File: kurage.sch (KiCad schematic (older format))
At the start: 106 parts, among them SW1 ESC, SW10 R, SW11 Y, SW12 I, SW13 P, SW14 ], SW15 UNDEFINED2, SW16 CTRL, SW17 A, SW18 D, SW19 G, SW2 Q, SW20 J, SW21 L, SW22 ', SW23 S, SW24 F, SW25 H, SW26 K, SW27 ;, SW28 ENTER, SW29 UNDEFINED3, SW3 E, SW30 LSHIFT, SW31 Z, SW32 C, SW33 B, SW34 M, SW35 ., SW36 RSHIFT, SW37 X, SW38 V, SW39 N, SW4 T, SW40 ,, SW41 /, SW42 UP, SW43 LOWER, SW44 UNDEFINED1, SW45 WIN, SW46 RAISE, SW47 LEFT, SW48 RIGHT, SW49 LSPACE, SW5 U, SW50 RSPACE, SW51 ALT, SW52 DOWN, SW6 O, SW7 [, SW8 BACKSPACE, SW9 W, U1 Elite-C

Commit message: progress
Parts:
- SW1, SW44, SW46: footprint MX_Only:MXOnly-1U-Hotswap -> MX_Only:MXOnly-1.5U-Hotswap
- SW16, SW8: footprint MX_Only:MXOnly-1U-Hotswap -> MX_Only:MXOnly-1.75U-Hotswap
- SW28, SW30: footprint MX_Only:MXOnly-1U-Hotswap -> MX_Only:MXOnly-2.25U-Hotswap
- SW36, SW49: footprint MX_Only:MXOnly-1U-Hotswap -> MX_Only:MXOnly-2U-Hotswap
- SW43: footprint MX_Only:MXOnly-1U-Hotswap -> MX_Only:MXOnly-1.25U-Hotswap
- SW50: footprint MX_Only:MXOnly-1U-Hotswap -> MX_Only:MXOnly-2.75U-Hotswap
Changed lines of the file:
@@
 F 0 "SW44" H 4600 4055 50  0000 C CNN
 F 1 "UNDEFINED1" H 4600 3964 50  0000 C CNN
-F 2 "MX_Only:MXOnly-1U-Hotswap" H 4600 3800 50  0001 C CNN
+F 2 "MX_Only:MXOnly-1.5U-Hotswap" H 4600 3800 50  0001 C CNN
 F 3 "" H 4600 3800 50  0000 C CNN
 	1    4600 3800
@@
 F 0 "SW49" H 4600 4455 50  0000 C CNN
 F 1 "LSPACE" H 4600 4364 50  0000 C CNN
-F 2 "MX_Only:MXOnly-1U-Hotswap" H 4600 4200 50  0001 C CNN
+F 2 "MX_Only:MXOnly-2U-Hotswap" H 4600 4200 50  0001 C CNN
 F 3 "" H 4600 4200 50  0000 C CNN
 	1    4600 4200
@@
 F 0 "SW46" H 6600 4055 50  0000 C CNN
 F 1 "RAISE" H 6600 3964 50  0000 C CNN
-F 2 "MX_Only:MXOnly-1U-Hotswap" H 6600 3800 50  0001 C CNN
+F 2 "MX_Only:MXOnly-1.5U-Hotswap" H 6600 3800 50  0001 C CNN
 F 3 "" H 6600 3800 50  0000 C CNN
 	1    6600 3800
@@
 F 0 "SW28" H 8600 2855 50  0000 C CNN
 F 1 "ENTER" H 8600 2764 50  0000 C CNN
-F 2 "MX_Only:MXOnly-1U-Hotswap" H 8600 2600 50  0001 C CNN
+F 2 "MX_Only:MXOnly-2.25U-Hotswap" H 8600 2600 50  0001 C CNN
 F 3 "" H 8600 2600 50  0000 C CNN
 	1    8600 2600
@@
 F 0 "SW36" H 8600 3255 50  0000 C CNN
 F 1 "RSHIFT" H 8600 3164 50  0000 C CNN
-F 2 "MX_Only:MXOnly-1U-Hotswap" H 8600 3000 50  0001 C CNN
+F 2 "MX_Only:MXOnly-2U-Hotswap" H 8600 3000 50  0001 C CNN
 F 3 "" H 8600 3000 50  0000 C CNN
 	1    8600 3000
@@
 F 0 "SW8" H 9600 1655 50  0000 C CNN
 F 1 "BACKSPACE" H 9600 1564 50  0000 C CNN
-F 2 "MX_Only:MXOnly-1U-Hotswap" H 9600 1400 50  0001 C CNN
+F 2 "MX_Only:MXOnly-1.75U-Hotswap" H 9600 1400 50  0001 C CNN
 F 3 "" H 9600 1400 50  0000 C CNN
 	1    9600 1400
@@
 F 0 "SW43" H 2600 4055 50  0000 C CNN
 F 1 "LOWER" H 2600 3964 50  0000 C CNN
-F 2 "MX_Only:MXOnly-1U-Hotswap" H 2600 3800 50  0001 C CNN
+F 2 "MX_Only:MXOnly-1.25U-Hotswap" H 2600 3800 50  0001 C CNN
 F 3 "" H 2600 3800 50  0000 C CNN
 	1    2600 3800
@@
 F 0 "SW30" H 2600 3255 50  0000 C CNN
 F 1 "LSHIFT" H 2600 3164 50  0000 C CNN
-F 2 "MX_Only:MXOnly-1U-Hotswap" H 2600 3000 50  0001 C CNN
+F 2 "MX_Only:MXOnly-2.25U-Hotswap" H 2600 3000 50  0001 C CNN
 F 3 "" H 2600 3000 50  0000 C CNN
 	1    2600 3000
@@
 F 0 "SW16" H 2600 2455 50  0000 C CNN
 F 1 "CTRL" H 2600 2364 50  0000 C CNN
-F 2 "MX_Only:MXOnly-1U-Hotswap" H 2600 2200 50  0001 C CNN
+F 2 "MX_Only:MXOnly-1.75U-Hotswap" H 2600 2200 50  0001 C CNN
 F 3 "" H 2600 2200 50  0000 C CNN
 	1    2600 2200
@@
 F 0 "SW1" H 2600 1655 50  0000 C CNN
 F 1 "ESC" H 2600 1564 50  0000 C CNN
-F 2 "MX_Only:MXOnly-1U-Hotswap" H 2600 1400 50  0001 C CNN
+F 2 "MX_Only:MXOnly-1.5U-Hotswap" H 2600 1400 50  0001 C CNN
 F 3 "" H 2600 1400 50  0000 C CNN
 	1    2600 1400
@@
 F 0 "SW50" H 5600 4455 50  0000 C CNN
 F 1 "RSPACE" H 5600 4364 50  0000 C CNN
-F 2 "MX_Only:MXOnly-1U-Hotswap" H 5600 4200 50  0001 C CNN
+F 2 "MX_Only:MXOnly-2.75U-Hotswap" H 5600 4200 50  0001 C CNN
 F 3 "" H 5600 4200 50  0000 C CNN
 	1    5600 4200

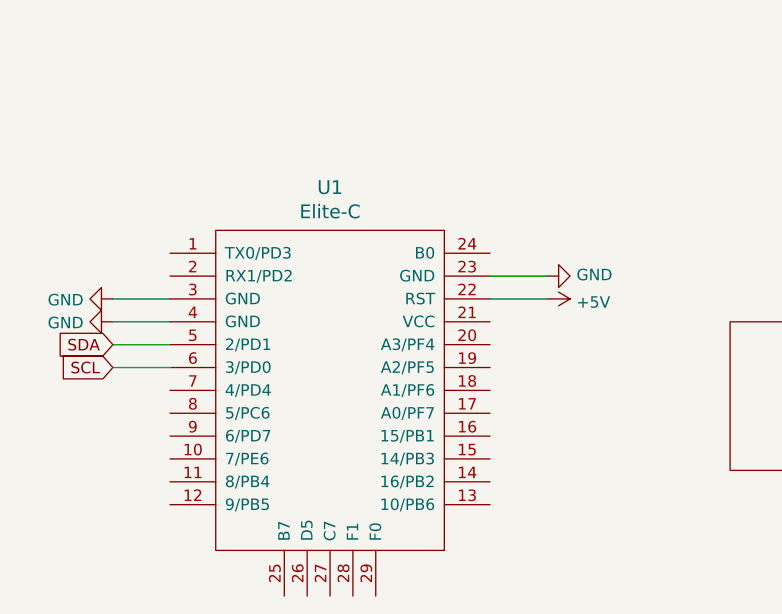
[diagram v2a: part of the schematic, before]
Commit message: save
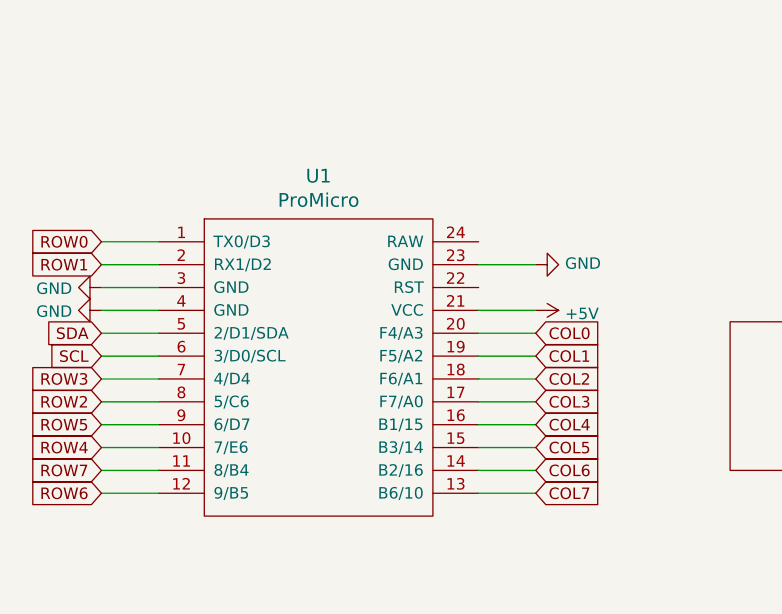
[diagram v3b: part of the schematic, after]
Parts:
- removed U1: Elite-C, Keebio-Parts:Elite-C, symbol keebio:Elite-C
- added U1: ProMicro, kbd:ProMicro_v3, symbol kbd:ProMicro
- SW10, SW11, SW12, SW13, SW14, SW15, SW17, SW18, SW19, SW2, SW20, SW21, SW22, SW23, SW24, SW25, SW26, SW27, SW29, SW3, SW31, SW32, SW33, SW34, SW35, SW37, SW38, SW39, SW4, SW40, SW41, SW42, SW45, SW47, SW48, SW5, SW51, SW52, SW6, SW7, SW9: footprint MX_Only:MXOnly-1U-Hotswap -> kbd:CherryMX_Hotswap
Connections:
- net +5V: now also U1.21 (VCC)
- net COL0: now also U1.20 (F4/A3)
- net COL1: now also U1.19 (F5/A2)
- net COL2: now also U1.18 (F6/A1)
- net COL3: now also U1.17 (F7/A0)
- net COL4: now also U1.16 (B1/15)
- net COL5: now also U1.15 (B3/14)
- net COL6: now also U1.14 (B2/16)
- net COL7: now also U1.13 (B6/10)
- net GND: now also U1.23 (GND), U1.3 (GND), U1.4 (GND)
- net ROW0: now also U1.1 (TX0/D3)
- net ROW1: now also U1.2 (RX1/D2)
- net ROW2: now also U1.8 (5/C6)
- net ROW3: now also U1.7 (4/D4)
- net ROW4: now also U1.10 (7/E6)
- net ROW5: now also U1.9 (6/D7)
- net ROW6: now also U1.12 (9/B5)
- net ROW7: now also U1.11 (8/B4)
- net SCL: now also U1.6 (3/D0/SCL)
- net SDA: now also U1.5 (2/D1/SDA)
